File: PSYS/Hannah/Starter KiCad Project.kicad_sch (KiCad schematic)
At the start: 0 parts

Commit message: mcu power and decoupling
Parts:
- added C1, C2, C3, C4, C5, C6: 100n, symbol Device:C
- added C7: 4u7, symbol Device:C
- added U1: STM32WB55CEUx, Package_DFN_QFN:QFN-48-1EP_7x7mm_P0.5mm_EP5.6x5.6mm, symbol MCU_ST_STM32WB:STM32WB55CEUx
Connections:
- new net +3.3V: C1.1, C2.1, C3.1, C4.1, C5.1, C6.1, C7.1, U1.1 (VBAT), U1.20 (VDD), U1.35 (VDD), U1.40 (VDDUSB), U1.48 (VDD), U1.8 (VDDA)
- new net GND: C1.2, C2.2, C3.2, C4.2, C5.2, C6.2, C7.2, U1.22 (VSSRF), U1.32 (VSSSMPS), U1.49 (VSS)

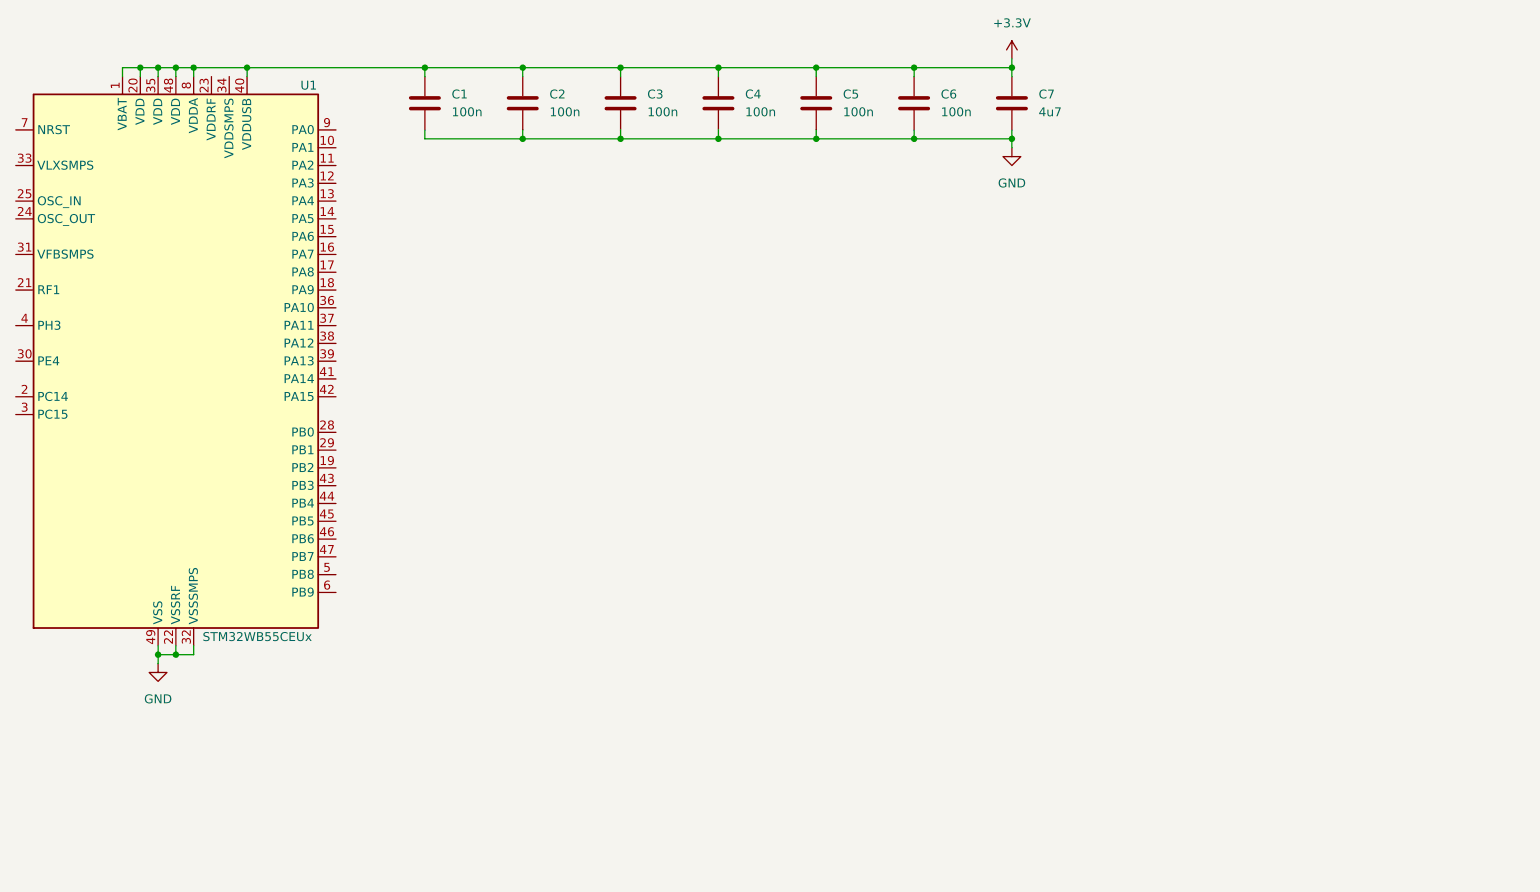
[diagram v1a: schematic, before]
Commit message: mcu smps
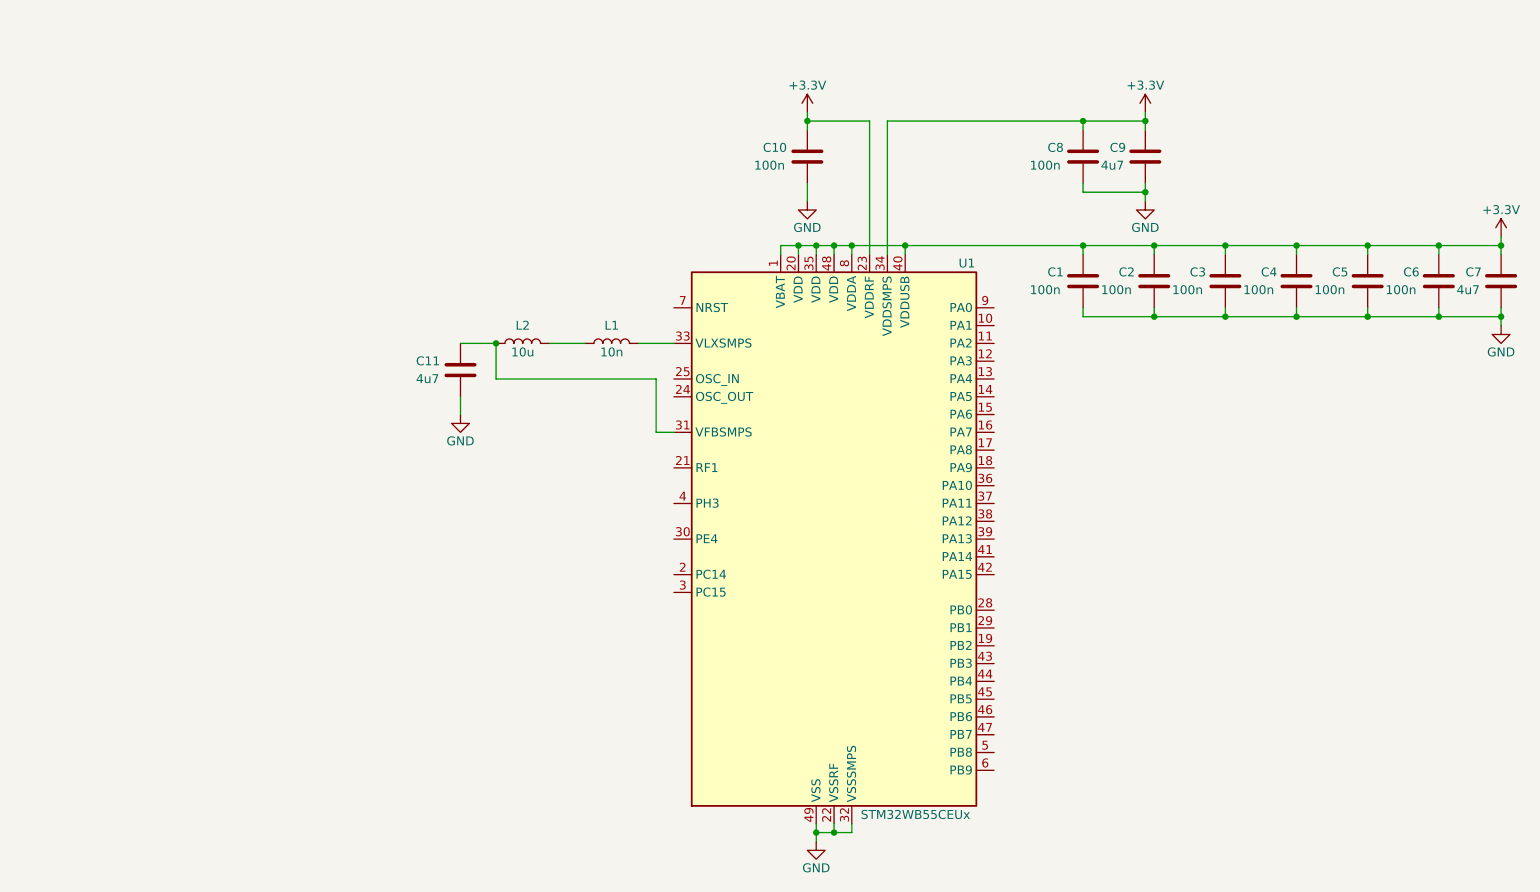
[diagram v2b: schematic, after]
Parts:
- added C10, C8: 100n, symbol Device:C
- added C11, C9: 4u7, symbol Device:C
- added L1: 10n, Package_SO:SOIC-8_3.9x4.9mm_P1.27mm, symbol Device:L
- added L2: 10u, Package_SO:SOIC-8_3.9x4.9mm_P1.27mm, symbol Device:L
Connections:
- net +3.3V: now also U1.23 (VDDRF), U1.34 (VDDSMPS), C10.1, C8.1, C9.1
- net GND: now also C10.2, C11.2, C8.2, C9.2
- net at U1.31 (VFBSMPS): now also C11.1, L2.1
- net at U1.33 (VLXSMPS): now also L1.2
- new net: L1.1, L2.2
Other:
- moved on the sheet: C1, C2, C3, C4, C5, C6, C7, U1
